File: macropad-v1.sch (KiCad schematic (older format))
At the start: 30 parts, among them J1 TYPE-C-31-M12_13, SW1 SW_Push, U1 ATmega32U4-AU, U2 USBLC6-2SC6, Y1 16MHz

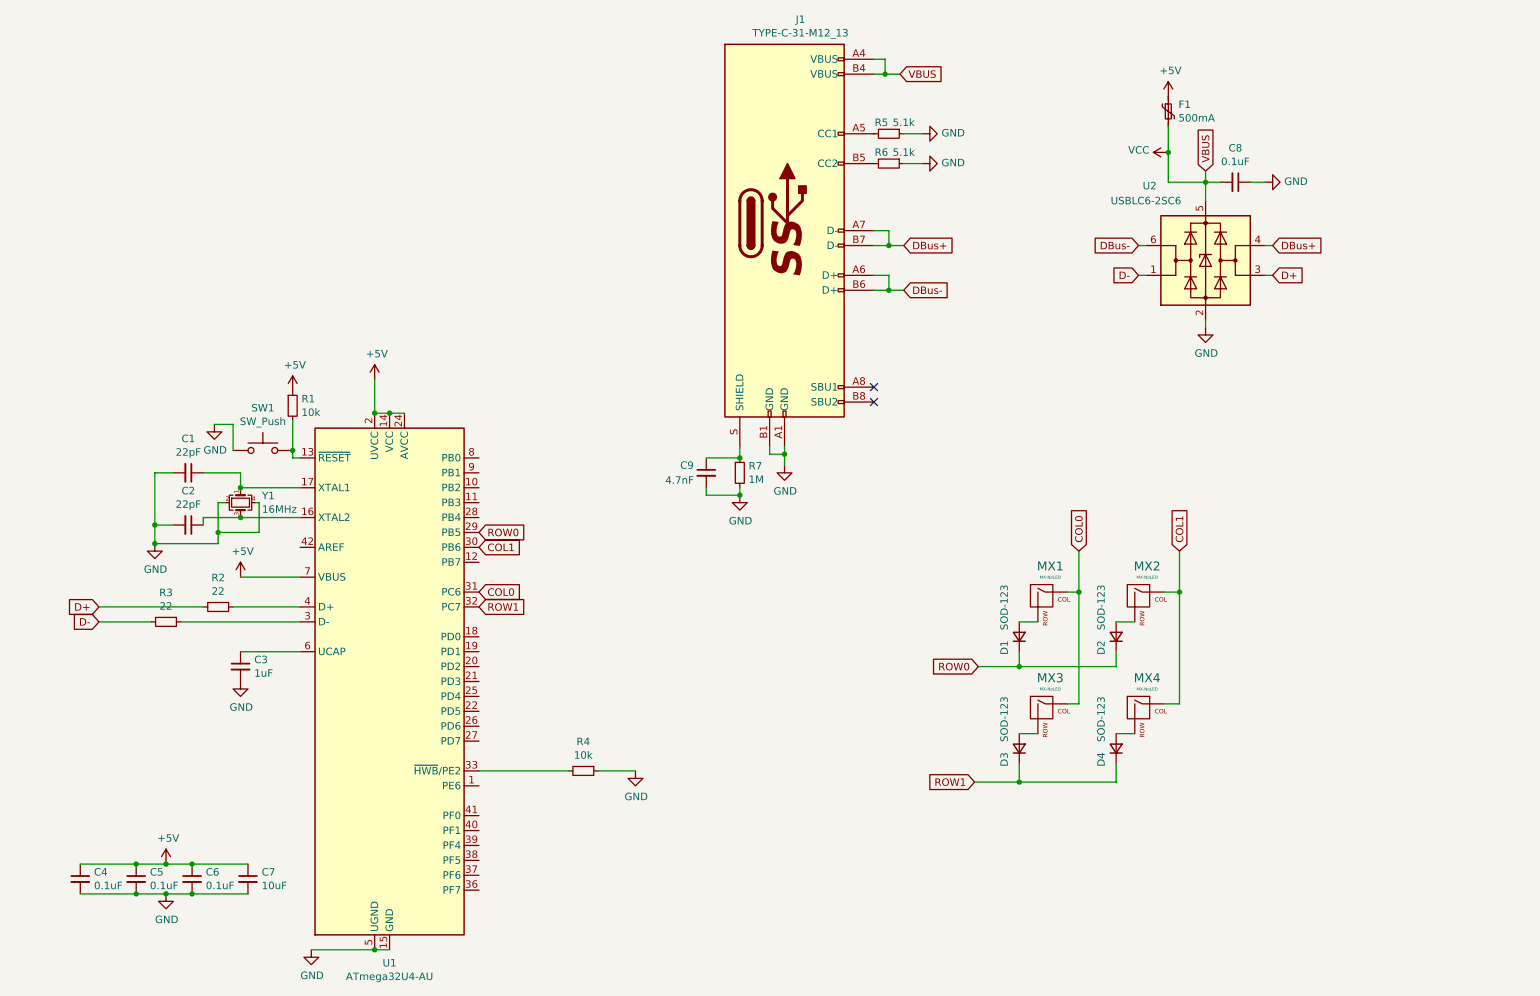
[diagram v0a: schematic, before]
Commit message: RGB
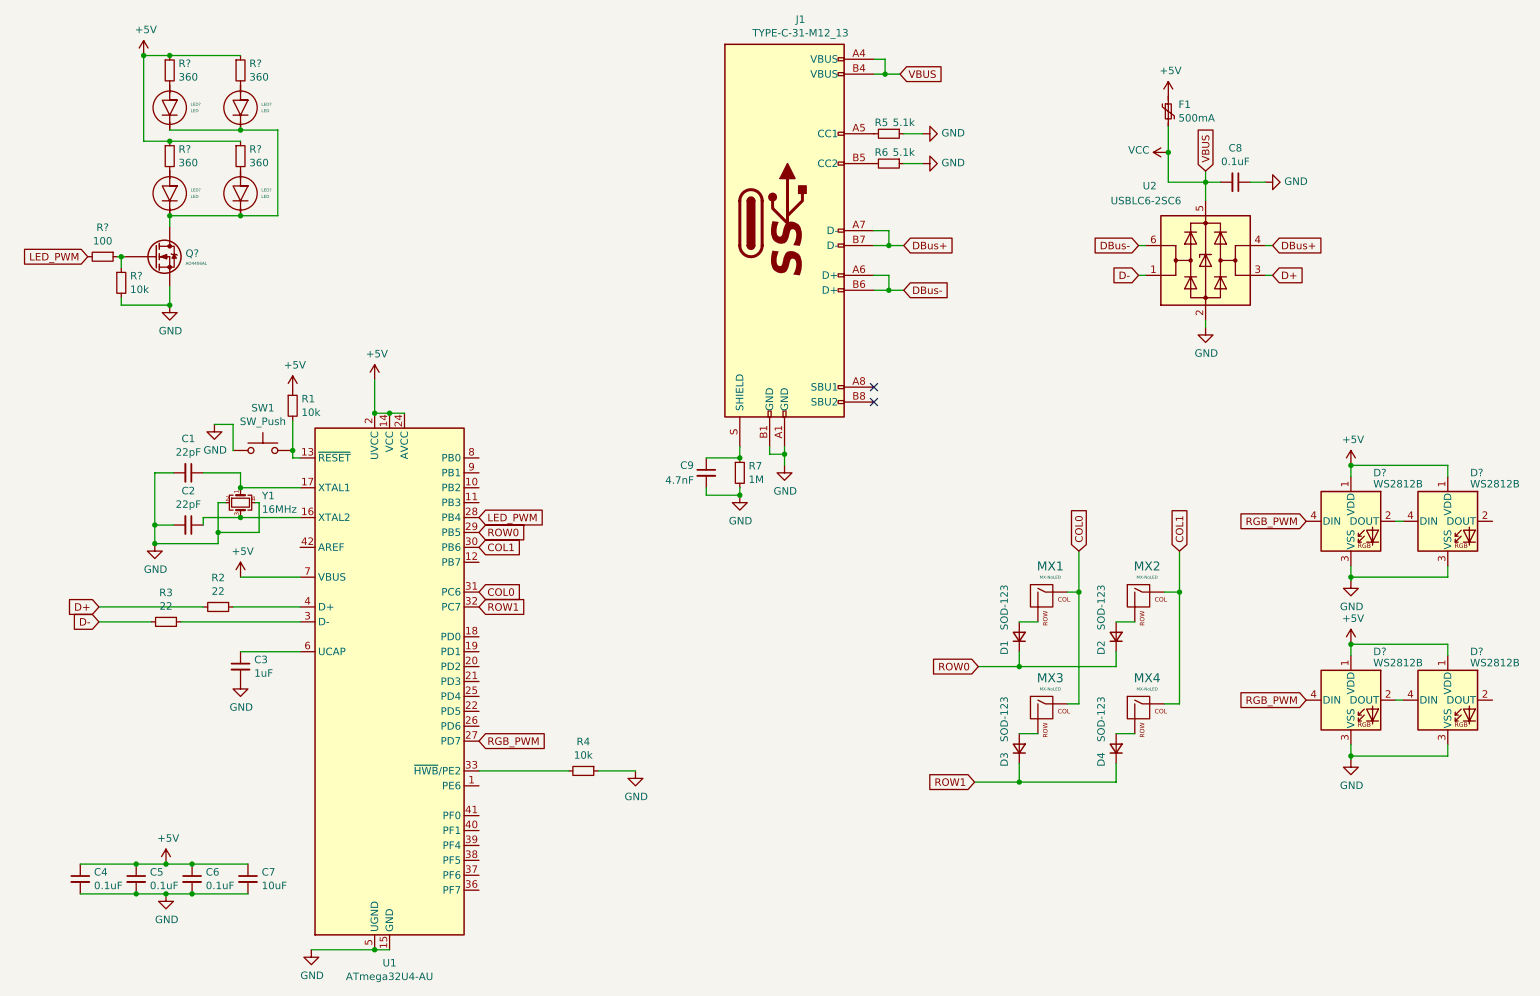
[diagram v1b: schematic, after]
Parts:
- added D? (x4): WS2812B, LED_SMD:LED_WS2812B_PLCC4_5.0x5.0mm_P3.2mm, symbol LED:WS2812B
- added LED? (x4): LED, symbol acheronSymbols:LED
- added Q?: AO4406AL, symbol acheronSymbols:AO4406AL
- added R? (x4): 360, symbol Device:R_Small
- added R?: 100, symbol Device:R_Small
- added R?: 10k, symbol Device:R_Small
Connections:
- net +5V: now also D?.1 (VDD), D?.1 (VDD), D?.1 (VDD), D?.1 (VDD), R?.1, R?.1, R?.1, R?.1
- net GND: now also D?.3 (VSS), D?.3 (VSS), D?.3 (VSS), D?.3 (VSS), Q?.1, Q?.2, Q?.3, R?.2
- net RGB_PWM: now reaches U1.27 (PD7)
- net RGB_PWM: now also D?.4 (DIN), D?.4 (DIN)
- net LED_PWM: now reaches U1.28 (PB4)
- net LED_PWM: now also R?.2
- new net: D?.2 (DOUT), D?.4 (DIN) (x2)
- new net: LED?.A, R?.2 (x4)
- new net: LED?.K, LED?.K, LED?.K, LED?.K, Q?.5 (D), Q?.6, Q?.7, Q?.8
- new net: Q?.4 (G), R?.1, R?.1
